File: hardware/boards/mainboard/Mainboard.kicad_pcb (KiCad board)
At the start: 2 copper layers, 118.1 x 101.6 mm, 117 parts, among them IC1 LM340?-MP, U1 CS42448, U2 PCA9536, U3 Breakoutboard

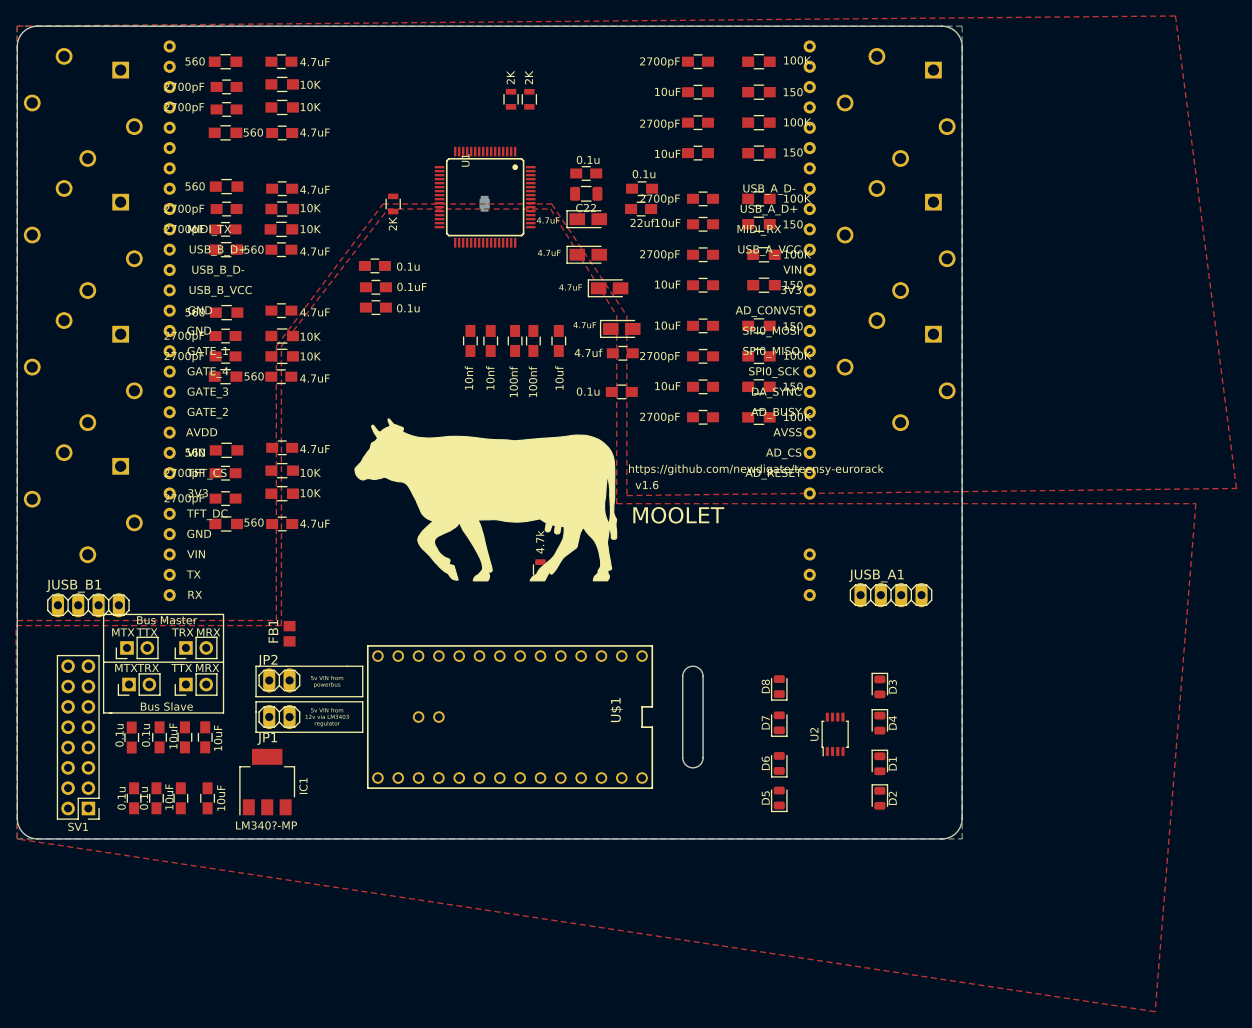
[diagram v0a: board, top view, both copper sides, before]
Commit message: mainboard v1.7 routed
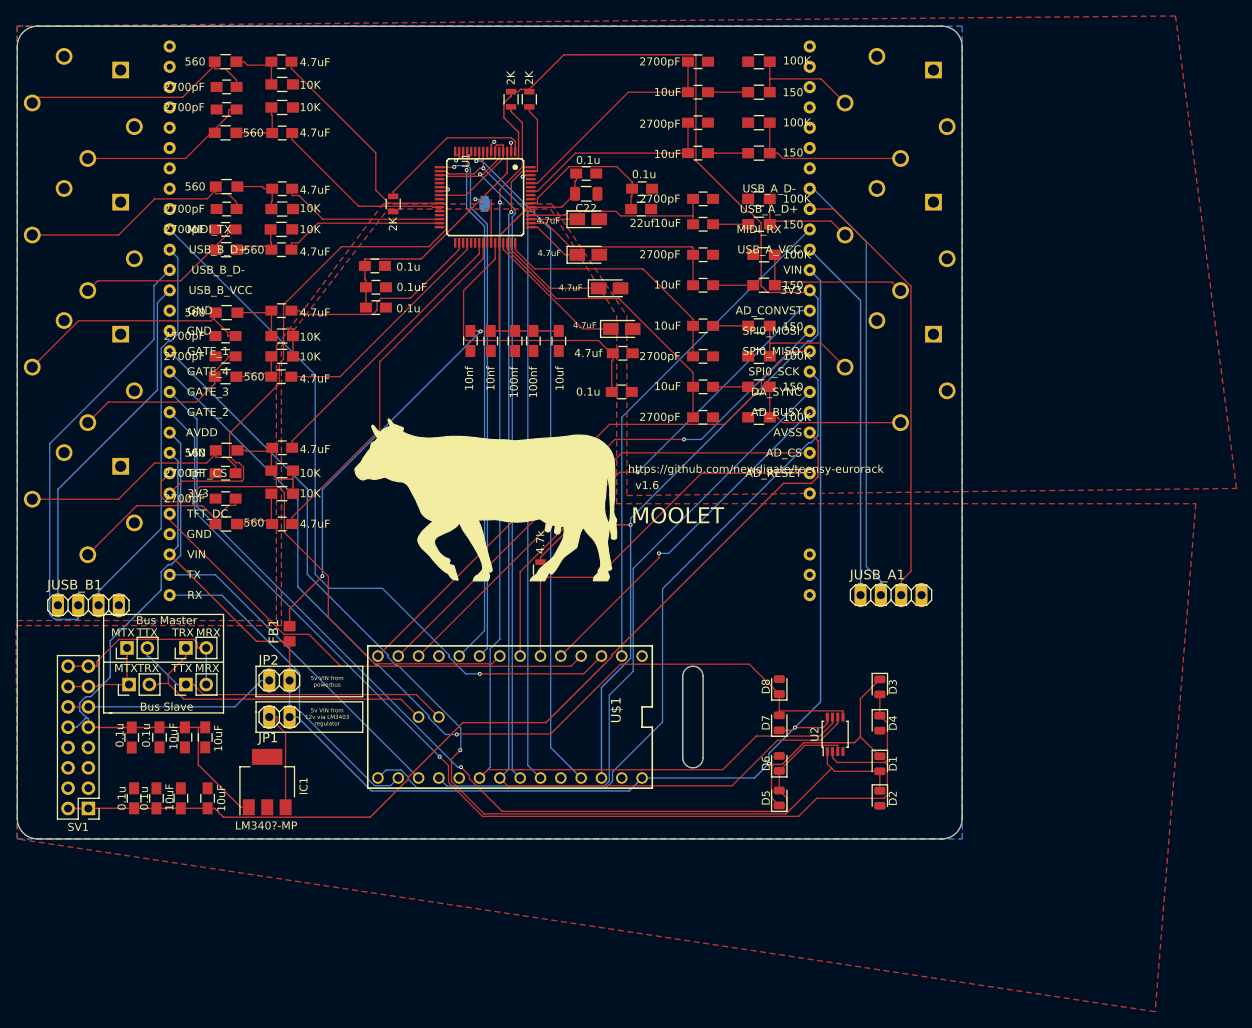
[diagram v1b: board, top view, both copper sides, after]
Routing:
- net VIN: track 0.00 -> 209.8 mm, vias 0 -> 2
- net +3V3: track 0.00 -> 192.5 mm, vias 0 -> 1
- net GATE_2: track 0.00 -> 139.2 mm, vias 0 -> 1
- net SDA: track 0.00 -> 135.5 mm, vias 0 -> 1
- net SCL: track 0.00 -> 134.0 mm, vias 0 -> 1
- net GATE_1: track 0.00 -> 132.0 mm, vias 0 -> 1
- net GATE_3: track 0.00 -> 120.2 mm, vias 0 -> 1
- net GATE_4: track 0.00 -> 118.1 mm, vias 0 -> 1
- net AVSS: track 0.00 -> 118.1 mm
- net SPI0_SCK: track 0.00 -> 93.7 mm
- net MIDI_TX: track 0.00 -> 92.7 mm, vias 0 -> 1
- net BCLK: track 0.00 -> 87.2 mm, vias 0 -> 1
- net LRCLK: track 0.00 -> 87.1 mm, vias 0 -> 1
- net MCLK: track 0.00 -> 84.3 mm, vias 0 -> 1
- net DA_SYNC: track 0.00 -> 81.0 mm
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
